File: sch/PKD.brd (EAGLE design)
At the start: 100 x 50 mm, 28 parts, among them IC1 LM393N, IC3 TL084P, IC4 74HC244N, Q2 BS170

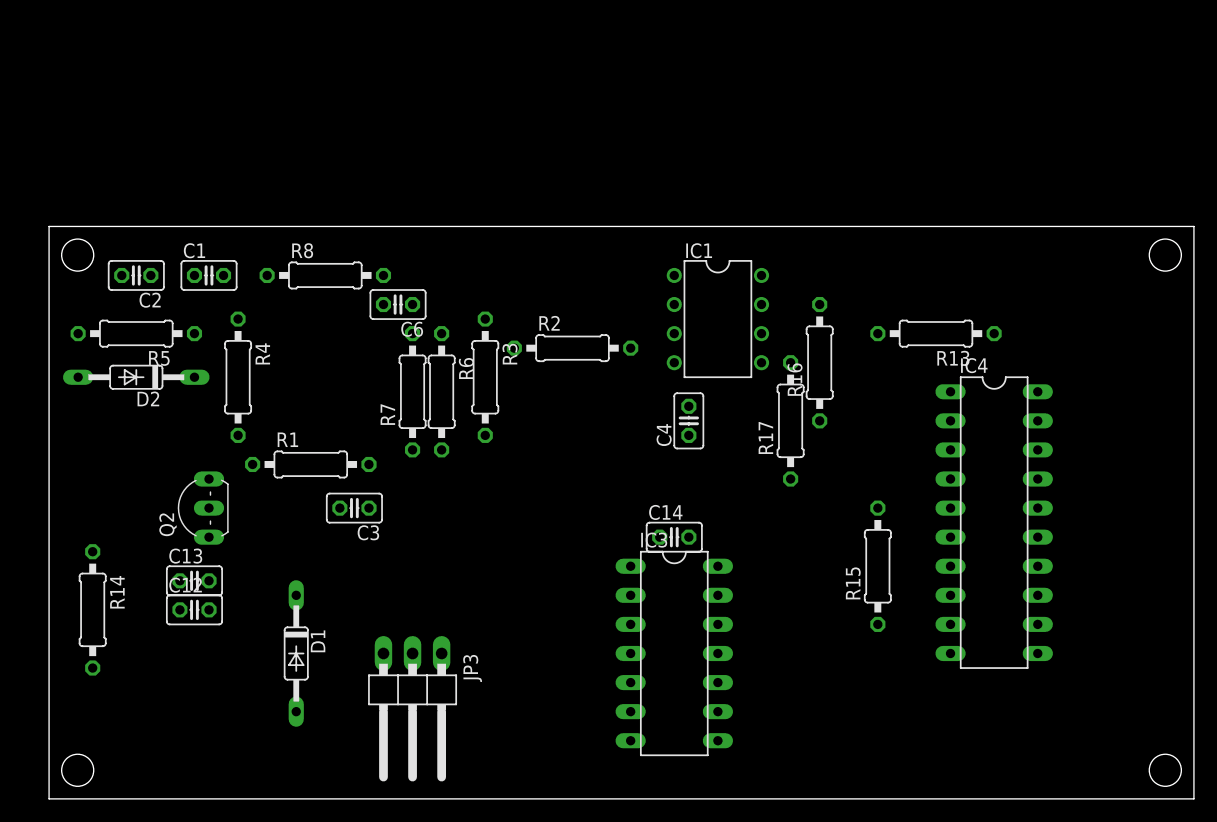
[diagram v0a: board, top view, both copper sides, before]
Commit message: BRD update
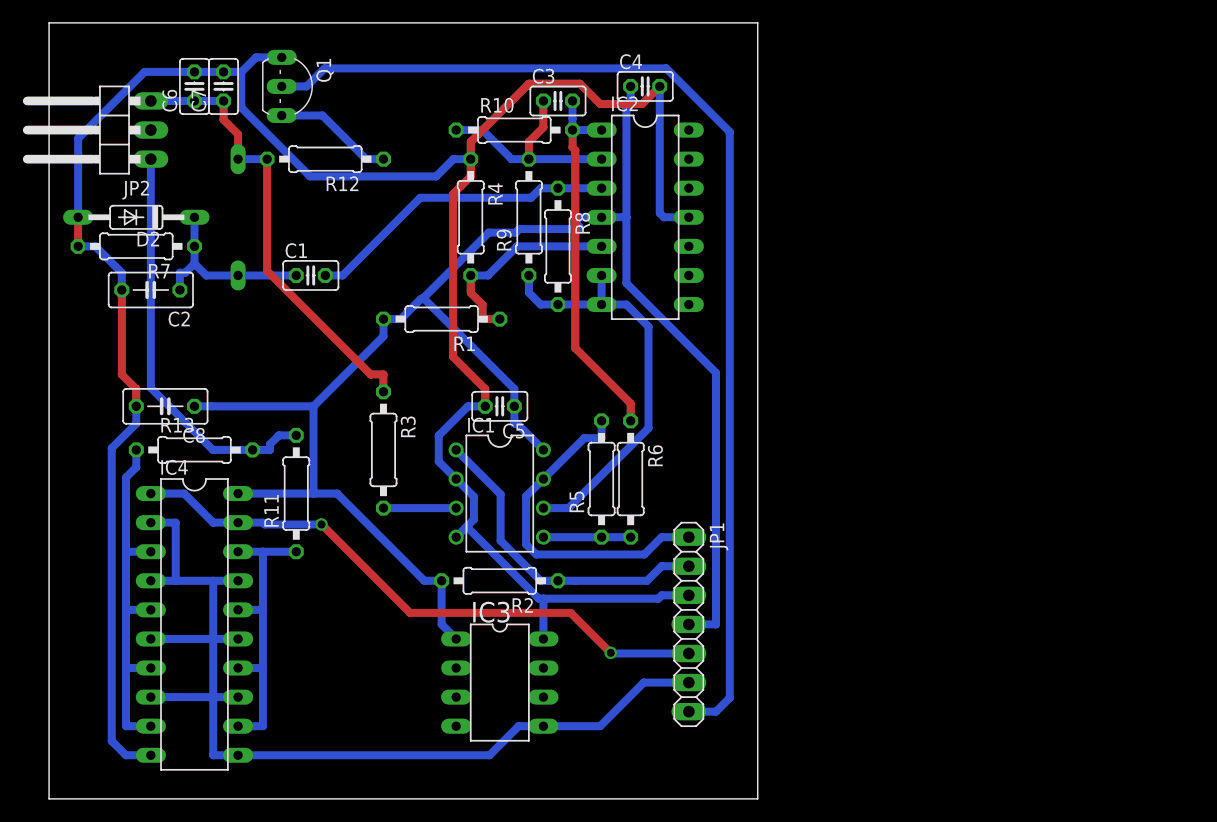
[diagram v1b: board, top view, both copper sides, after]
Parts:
- removed C12: 1n, rcl:C025-025X050
- removed C13: 2n2, rcl:C025-025X050
- removed C14: 33n, rcl:C025-025X050
- removed JP3: (no value), pinhead:1X03/90
- removed Q2: BS170, adam:TO92-
- removed R14: 220, rcl:0207/10
- removed R15: 33, rcl:0207/10
- removed R16: 10k, rcl:0207/10
- removed R17: 2,2k, rcl:0207/10
- added C5: 33n, rcl:C025-025X050
- added C7: 2n2, rcl:C025-025X050
- added C8: 33n, rcl:C050-030X075
- added IC2: TL084P, linear:DIL14
- added JP1: (no value), pinhead:1X07
- added JP2: (no value), pinhead:1X03/90
- added Q1: BS170, adam:TO92-
- added R10: 100k, rcl:0207/10
- added R11: 33, rcl:0207/10
- added R12: 220, rcl:0207/10
- added R9: 10k, rcl:0207/10
- C2: device rcl:C025-025X050 -> rcl:C050-030X075
- C3: value 33n -> 100p
- C6: value 100p -> 1n
- IC3: value TL084P -> PIC12F683P; device linear:DIL14 -> microchip:DIL8
- R5: value 510k -> 10k
- R6: value 100k -> 2,2k
- R7: value 10k -> 510k
- moved IC4 70.4 mm to (12.7, 15.2)
- moved R13 65.6 mm to (12.7, 30.5), turned to 0 degrees
- moved R5 42.6 mm to (48.3, 27.9), turned to 90 degrees
- moved C3 39.8 mm to (44.5, 61.0), turned to 0 degrees
- moved D1 38.4 mm to (16.5, 50.8), flipped to the bottom, turned to 90 degrees
- moved C4 29.5 mm to (52.1, 62.2), turned to 0 degrees
- moved R7 27.3 mm to (7.62, 48.3), turned to 180 degrees
- moved C6 26.1 mm to (12.7, 62.2), turned to 90 degrees
- moved R4 24.7 mm to (36.8, 50.8)
- moved IC1 24.4 mm to (39.4, 26.7)
- moved R2 21.3 mm to (39.4, 19.1), turned to 180 degrees
- moved R8 20.5 mm to (44.5, 48.3), turned to 270 degrees
- moved R6 18.2 mm to (50.8, 27.9)
- moved R1 17.1 mm to (34.3, 41.9), turned to 180 degrees
- moved IC3 15.5 mm to (39.4, 10.2)
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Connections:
- removed net PWR_OE2: IC4.19
- net ANT_LO: now also C6.1, C7.1, JP2.3, R12.2; no longer C12.1, C13.1, JP3.3, R14.2
- net CROSS_LO: now also JP1.2
- net GND: now also C5.2, C6.2, C7.2, C8.2, IC2.11, IC3.8, JP1.3, Q1.3, R7.2; no longer C12.2, C13.2, C14.2, C3.2, IC3.11, Q2.3, R5.2
- net LO_LOAD: now also JP1.7, Q1.2; no longer Q2.2
- net LO_PKD: now also JP1.1, R5.2; no longer R16.2
- net LO_PKD_U: now also C3.2, IC2.1, R10.2, R6.1; no longer C6.2, IC3.1, R17.1, R8.2
- net N$1: now also R7.1; no longer R5.1
- net N$13: now also JP2.1, R11.2; no longer JP3.1, R15.2
- net N$14: now also R11.1; no longer R13.1
- net N$15: now also R13.1; no longer R15.1
- net N$17: now also R5.1, R6.2; no longer R16.1, R17.2
- net N$2: now also IC2.3, R8.1; no longer IC3.3, R6.1
- net N$3: now also IC2.5; no longer IC3.5
- net N$4: now also Q1.1, R12.1; no longer Q2.1, R14.1
- net N$5: now also C3.1, IC2.2, R10.1, R9.2; no longer C6.1, IC3.2, R7.2, R8.1
- net PWR_LO: now also IC3.5, JP1.6
- net PWR_OE1: now also IC4.19, JP1.5
- net VCC: now also C5.1, C8.1, IC2.4, IC3.1, JP1.4; no longer C14.1, C3.1, IC3.4
- net VMID: now also IC2.6, IC2.7, R8.2, R9.1; no longer IC3.6, IC3.7, R6.2, R7.1
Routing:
- net GND: track 0.00 -> 207.6 mm
- net VCC: track 0.00 -> 151.0 mm
- net LO_LOAD: track 0.00 -> 95.6 mm
- net PWR_LO: track 0.00 -> 89.5 mm
- net PWR_OE1: track 0.00 -> 52.8 mm, vias 0 -> 2
- net ANT_LO: track 0.00 -> 39.7 mm
- net VMID: track 0.00 -> 36.7 mm
- net N$13: track 0.00 -> 35.7 mm
- net N$15: track 0.00 -> 33.2 mm
- net LO_PKD_U: track 0.00 -> 32.6 mm
- net LO_PKD: track 0.00 -> 29.6 mm
- net CROSS_LO: track 0.00 -> 28.0 mm
- net N$2: track 0.00 -> 27.3 mm
- net N$14: track 0.00 -> 26.8 mm
- net N$5: track 0.00 -> 19.4 mm
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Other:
- board size 100 x 50 mm -> 61.9 x 67.8 mm

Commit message: Added pic12f firmware and updated schematic
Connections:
- new net BIT_IN: IC3.3
- new net OCLK: IC3.6
- net CROSS_LO: now also IC3.2
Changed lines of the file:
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@@
 <?xml version="1.0" encoding="utf-8"?>
 <!DOCTYPE eagle SYSTEM "eagle.dtd">
-<eagle version="6.2">
+<eagle version="6.1">
 <drawing>
 <settings>
@@
 <wire x1="39.4398" y1="26.6002" x2="39.4398" y2="22.5497" width="0.7" layer="16"/>
 <wire x1="39.4398" y1="22.5497" x2="42.9395" y2="19.05" width="0.7" layer="16"/>
+<contactref element="IC3" pad="2"/>
+<wire x1="35.56" y1="11.43" x2="42.9395" y2="19.05" width="0" layer="19" extent="16-16"/>
 </signal>
 <signal name="ANT_LO">
@@
 <wire x1="11.7991" y1="26.67" x2="8.89" y2="26.67" width="0.7" layer="16"/>
 </signal>
+<signal name="OCLK">
+<contactref element="IC3" pad="6"/>
+</signal>
+<signal name="BIT_IN">
+<contactref element="IC3" pad="3"/>
+</signal>
 </signals>

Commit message: First emulator function - not working
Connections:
- new net NRST: IC3.4
- new net R/E: IC3.7
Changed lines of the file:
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@@
 <contactref element="IC3" pad="3"/>
+</signal>
+<signal name="R/E">
+<contactref element="IC3" pad="7"/>
+</signal>
+<signal name="NRST">
+<contactref element="IC3" pad="4"/>
 </signal>
 </signals>
